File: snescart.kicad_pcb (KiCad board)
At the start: 2 copper layers, 101.6 x 37.3 mm, 7 parts, among them P1 CASSETTE, U1 27C080

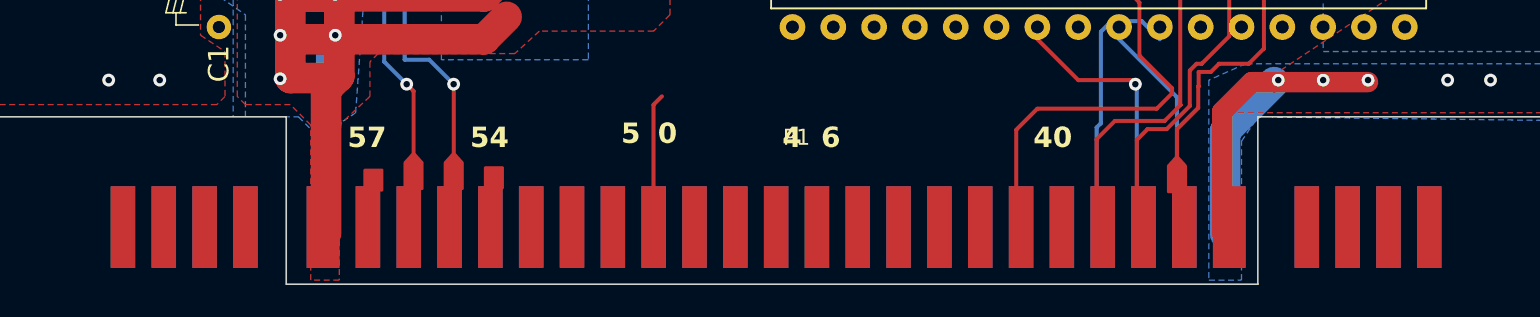
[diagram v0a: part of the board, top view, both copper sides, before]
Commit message: 38mil spacing smh
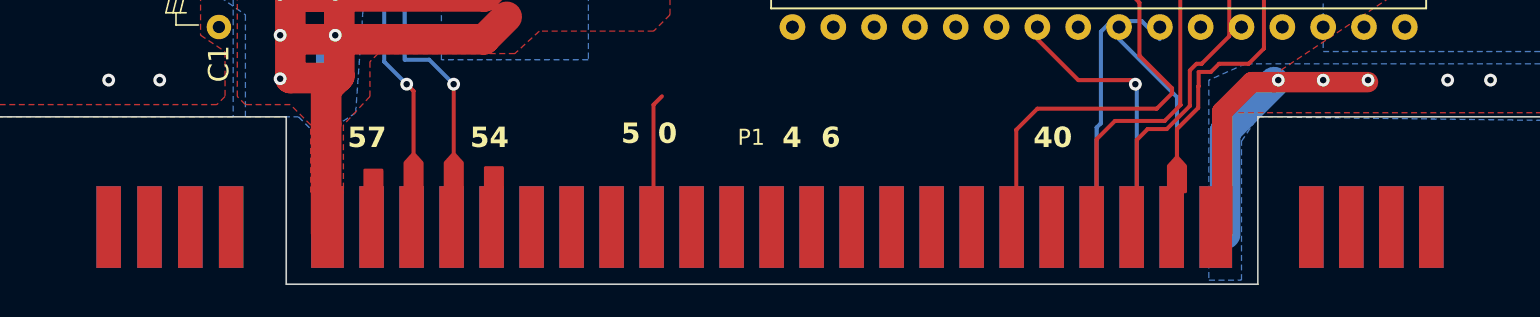
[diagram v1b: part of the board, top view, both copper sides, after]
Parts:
- moved P1 2.82 mm to (143.5, 143.8)
